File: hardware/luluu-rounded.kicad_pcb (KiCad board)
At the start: 4 copper layers, 64 x 30 mm, 71 parts, among them J1 BATT_CON, J2 RPi SWD, J3 STEMMA_{QT} I_{2}C, J4 Micro_SD_Card, J5 GPIO0, J6 USB_C_Receptacle_USB2.0, J7 DISP_LCD_ST7789, J8 GPIO1, Q1 AO3401A, Q2 BSS138, SW1 SW_B, SW2 SW_A, SW3 SW_POWER, U1 W25Q128JVSS, U2 RT9080-33GJ5, U3 RP2040, U4 TP4054-42, U5 LIS3DH, Y1 X322512MSB4SI

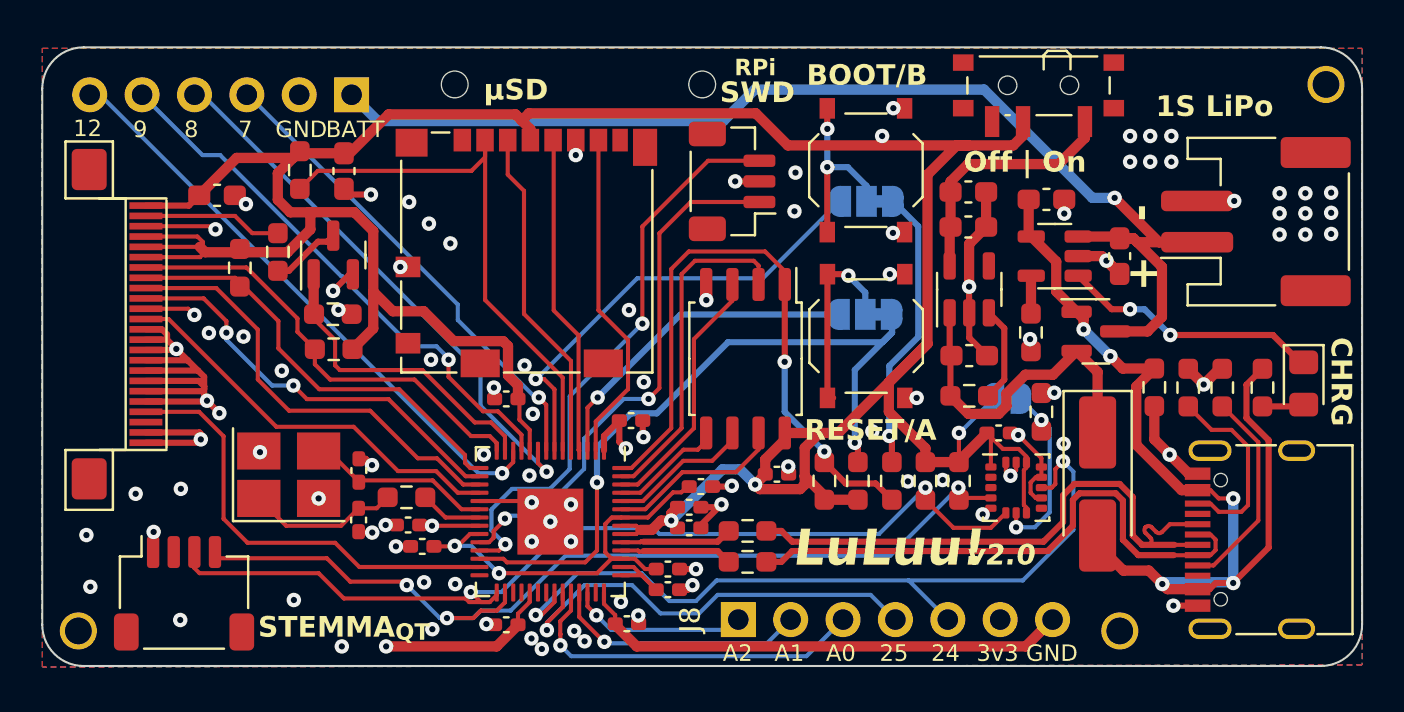
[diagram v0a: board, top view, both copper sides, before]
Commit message: 2.0 release candidate
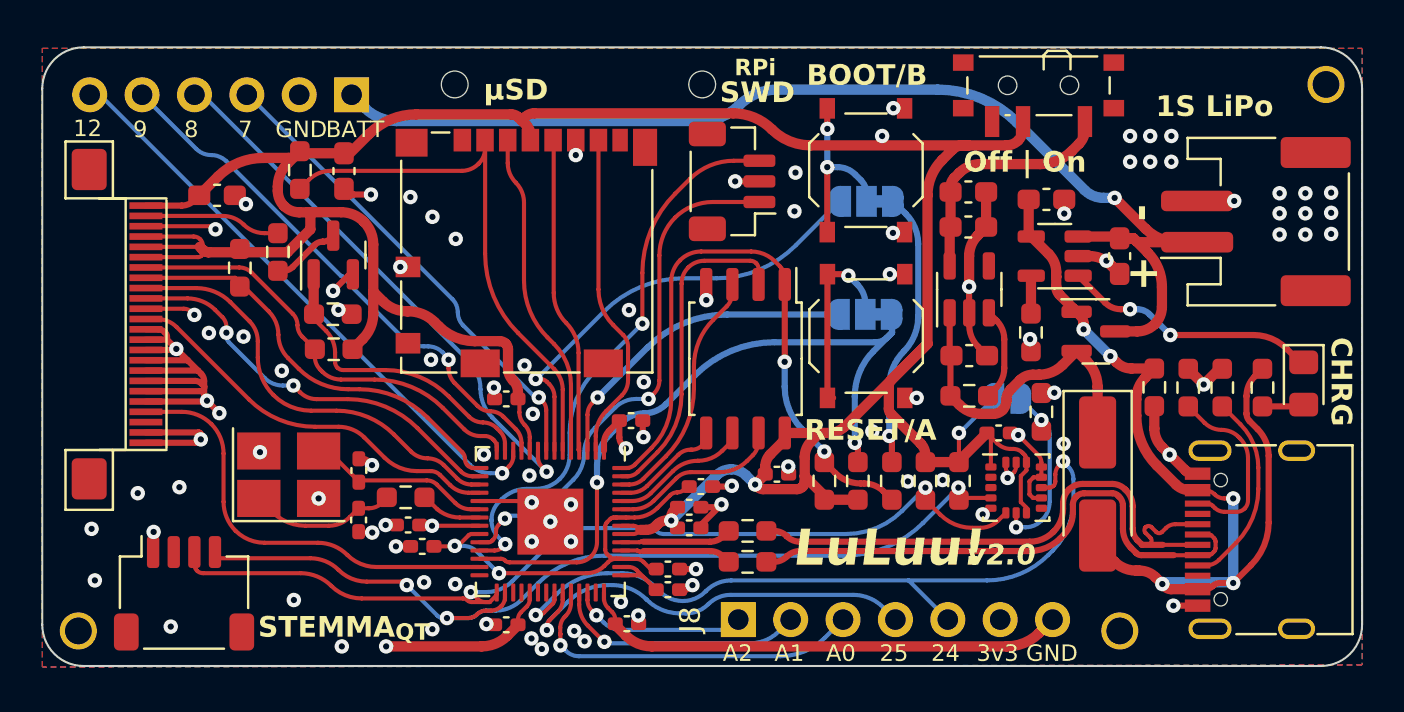
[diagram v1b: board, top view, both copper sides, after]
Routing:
- net +3V3: track 196.2 -> 193.0 mm
- net /I_{2}C_{CLOCK}: track 46.0 -> 44.8 mm
- net +5V: track 49.0 -> 47.9 mm
- net +BATT: track 58.7 -> 57.7 mm
- net /GPIO_D24: track 38.8 -> 37.7 mm
- net /SWD: track 28.2 -> 27.2 mm
- net /SW_A_RST: track 35.6 -> 34.8 mm
- net /I_{2}C_{DATA}: track 47.2 -> 46.4 mm
- net /DISP_SPI_{CLOCK}: track 21.5 -> 20.8 mm
- net Net-(U1-~{CS}): track 31.3 -> 30.6 mm
- net /GPIO_D25: track 21.6 -> 20.9 mm
- net /DISP_~{CS_{MAIN}}: track 21.0 -> 20.4 mm
- net /SW_B_GPIO: track 22.4 -> 21.8 mm
- net /DISP_VSYNC: track 21.6 -> 21.1 mm
- net /SWD_{CLOCK}: track 25.9 -> 25.3 mm
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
